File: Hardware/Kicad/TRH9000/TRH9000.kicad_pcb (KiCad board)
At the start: 4 copper layers, 99.1 x 77.2 mm, 68 parts, among them J1 RGB, J2 RGB, Q1 BC817, SW1 SW_DP3T, U1 74HC138, U2 74HC32, U3 V9990, U4 KM428C256, U5 KM428C256, U6 LMH1980, U7 ICL7660, U8 LT1675, X1 14.31818MHz, Y1 21.47727Mhz

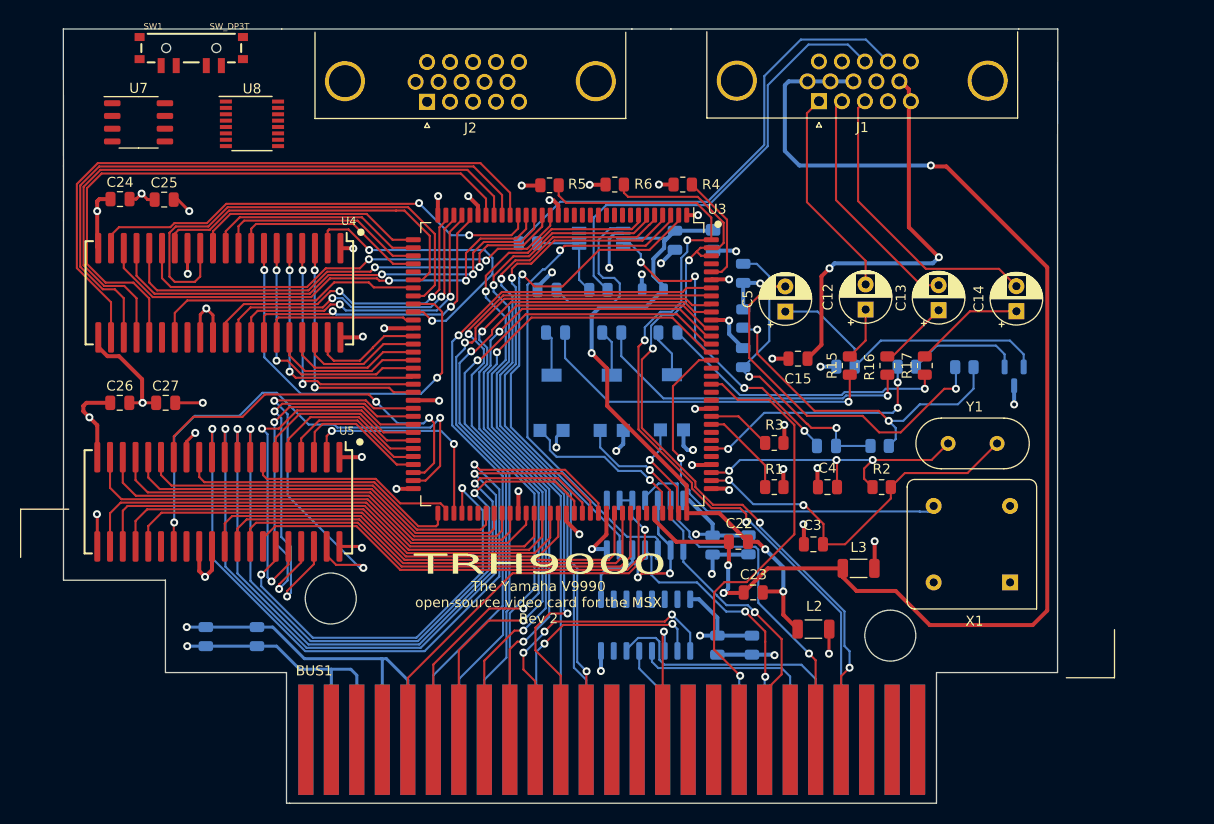
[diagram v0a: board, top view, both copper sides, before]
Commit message: Multiple changes.
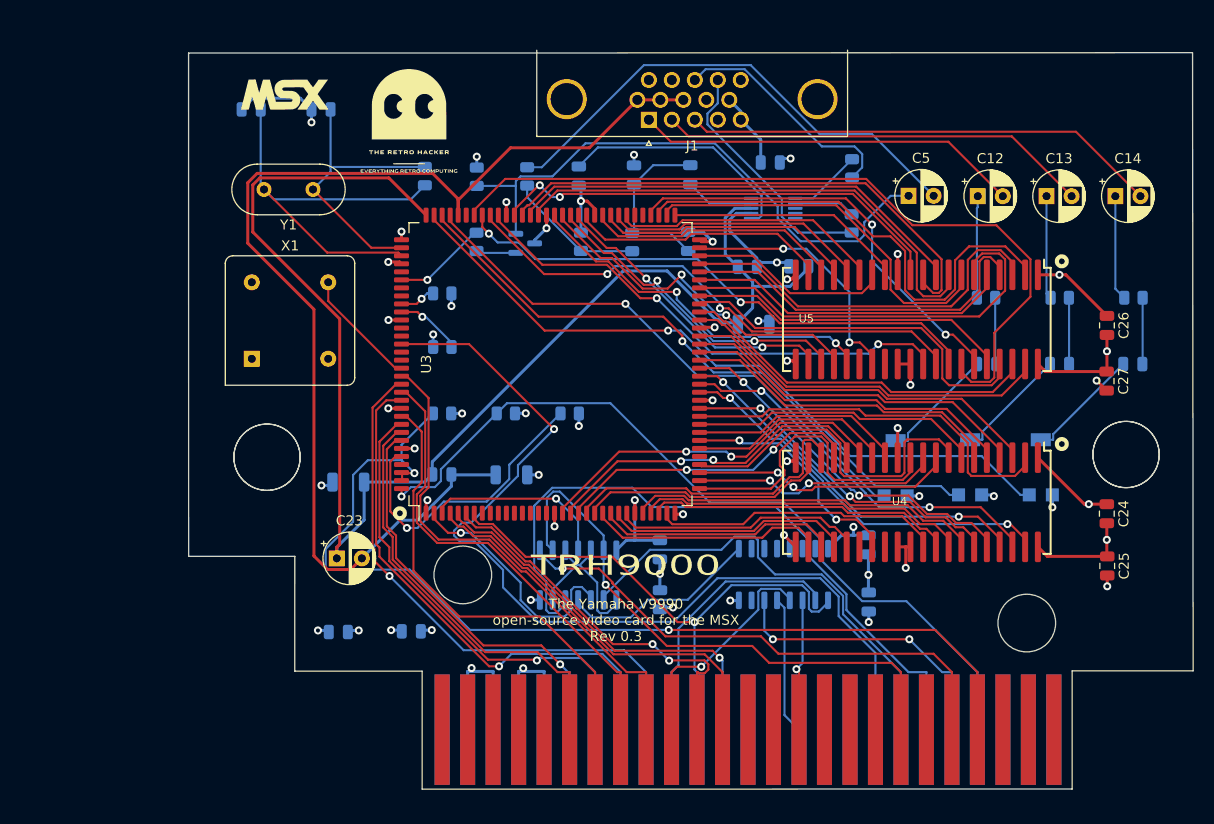
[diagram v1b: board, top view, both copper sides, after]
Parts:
- removed Cart1: MSX-cartridge_dummy, trh9000:MSX-cart-dummy
- removed J2: RGB, Connector_Dsub:DSUB-15-HD_Female_Horizontal_P2.29x1.98mm_EdgePinOffset3.03mm_Housed_MountingHolesOffset4.94mm
- removed SW1: SW_DP3T, Switches:SWITCH_SP3T_SMD
- removed U7: ICL7660, Package_SO:SOP-8_3.9x4.9mm_P1.27mm
- removed U8: LT1675, Package_SO:SSOP-16_3.9x4.9mm_P0.635mm
- C15, C22, C3, C4, L2, L3, R1, R15, R16, R17, R2, R3, R4, R5, R6: moved to B.Cu
- C16: footprint Capacitor_SMD:C_0805_2012Metric_Pad1.18x1.45mm_HandSolder -> Capacitor_SMD:C_0805_2012Metric
- C23: footprint Capacitor_SMD:C_0805_2012Metric -> Capacitor_THT:CP_Radial_D5.0mm_P2.50mm
- L1: footprint Inductor_SMD:L_0805_2012Metric -> Inductor_SMD:L_1206_3216Metric
- MSX1, TRH1: renamed from G***; moved to F.Cu
- moved C24 103.2 mm to (202.2, 98.2), turned to -90 degrees
- moved C25 100.8 mm to (202.3, 103.4), turned to -90 degrees
- moved C26 98.7 mm to (202.2, 79.4), turned to -90 degrees
- moved C27 93.8 mm to (202.2, 84.9), turned to -90 degrees
- moved X1 78.8 mm to (117.0, 82.7), turned to 0 degrees
- moved Y1 72.7 mm to (123.1, 65.8)
- moved U4 72.6 mm to (183.3, 97.0)
- moved U5 71.9 mm to (183.3, 78.8)
- moved C4 68.7 mm to (117.0, 57.9)
- moved C3 65.5 mm to (123.9, 57.9)
- moved R2 55.1 mm to (134.3, 64.5), turned to 90 degrees
- moved Q1 50.5 mm to (144.3, 71.2), turned to 0 degrees
- moved L2 48.6 mm to (126.7, 95.0), turned to 0 degrees
- moved R9 47.5 mm to (144.5, 64.5), turned to 90 degrees
- moved C8 46.4 mm to (204.8, 83.2)
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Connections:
- U1 pad 1: /A4 -> /A3
- U1 pad 4: /~{IORQ} -> /A4
- U1 pad 9: Net-(U1-Pad9) -> Net-(U2-Pad4)
- U2 pad 1: /~{RD} -> Net-(U2-Pad1)
- U2 pad 10: /SYS_CLK -> Net-(U2-Pad1)
- U2 pad 11: /~{BUSDIR} -> /VDP/~{VDPR}
- U2 pad 12: Net-(U1-Pad9) -> Net-(U2-Pad1)
- U2 pad 2: Net-(U1-Pad9) -> /~{WR}
- U2 pad 3: /VDP/~{VDPR} -> /VDP/~{VDPW}
- U2 pad 4: /~{WR} -> Net-(U2-Pad4)
- U2 pad 5: Net-(U1-Pad9) -> /~{IORQ}
- U2 pad 6: /VDP/~{VDPW} -> Net-(U2-Pad1)
- U2 pad 8: /SCIN -> /~{BUSDIR}
- U2 pad 9: /SYS_CLK -> /~{RD}
- U4 pad 12: /VDP/~{V0_WE} -> GND
- U4 pad 13: GND -> /VDP/~{V0_WE}
- U5 pad 12: /VDP/~{V1_WE} -> GND
- U5 pad 13: GND -> /VDP/~{V1_WE}
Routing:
- net +5VA: track 69.0 -> 139.4 mm, vias 3 -> 0
- net /VDP/B: track 9.89 -> 71.1 mm
- net /VDP/G: track 12.7 -> 63.6 mm
- net /~{RESET}: track 47.0 -> 94.2 mm
- net /~{IORQ}: track 21.8 -> 68.8 mm
- net /SYS_CLK: track 42.2 -> 0.00 mm, vias 1 -> 0
- net /VDP/V0A3: track 64.2 -> 23.5 mm
- net GND: track 150.9 -> 111.6 mm, vias 36 -> 34
- net /VDP/V0A2: track 62.9 -> 23.9 mm
- net /VDP/R: track 17.4 -> 55.2 mm
- net /VDP/V0A1: track 62.2 -> 24.4 mm
- net /VDP/V0A0: track 61.4 -> 24.9 mm
- net /D6: track 76.7 -> 42.1 mm, vias 2 -> 0
- net /VDP/V1D7: track 44.8 -> 78.5 mm
- net /A2: track 71.8 -> 38.2 mm
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- added copper zone on In1.Cu, net +5V
- added copper zone on In2.Cu, net GND
- removed copper zone on In2.Cu, net +5V
- removed copper zone on In1.Cu, net GND
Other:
- board size 99.1 x 77.2 mm -> 100.1 x 73.4 mm
- board text added: "The Yamaha V9990 open-source video card for the MSX Rev 0.3"
- board text removed: "Designed by the MSX community for the MSX community."
- board text removed: "The Yamaha V9990 open-source video card for the MSX Rev 2"
